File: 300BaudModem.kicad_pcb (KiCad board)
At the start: 4 copper layers, 160 x 100 mm, 27 parts, among them U1 LM7905, X2 Raw

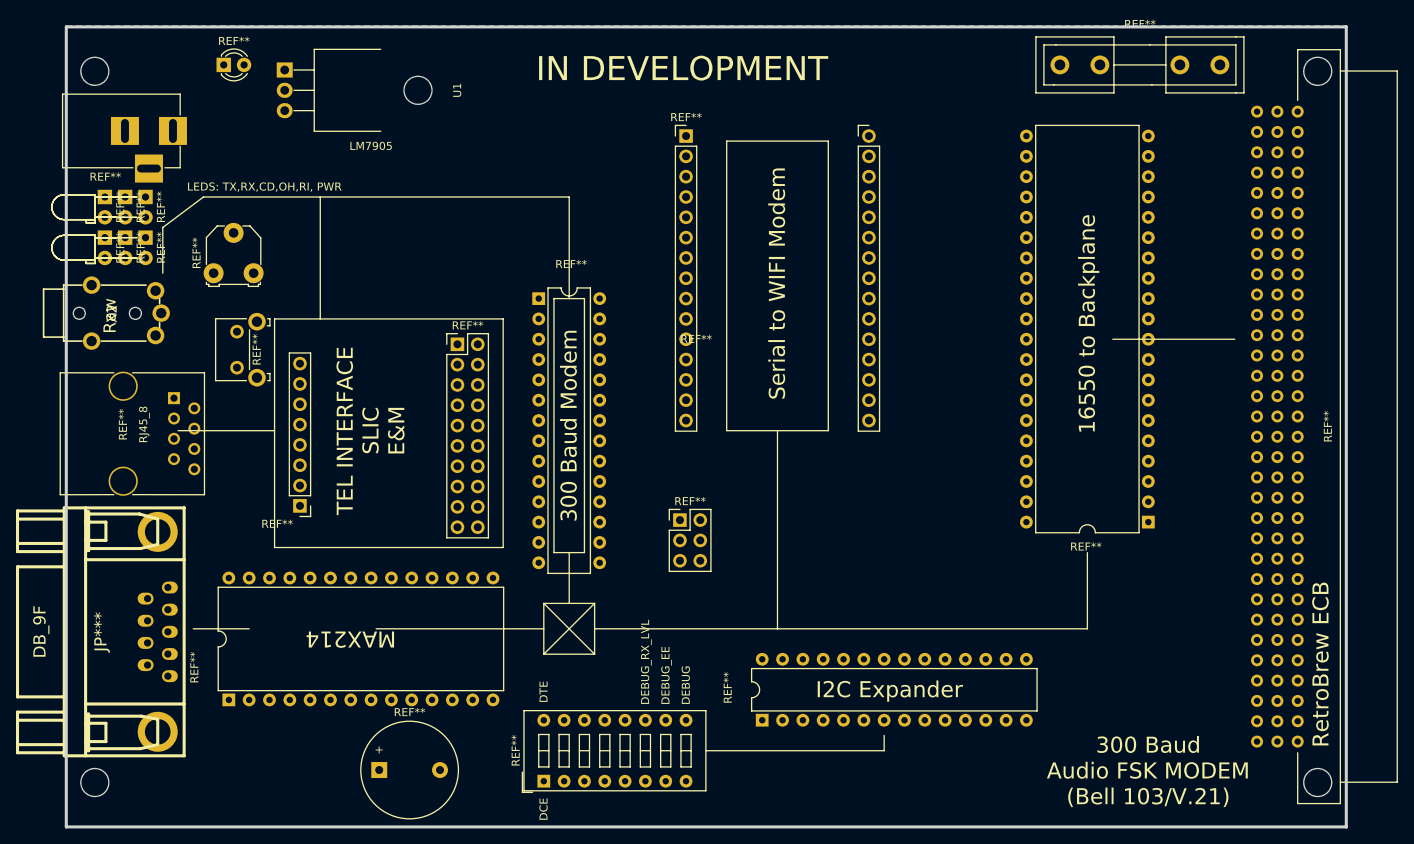
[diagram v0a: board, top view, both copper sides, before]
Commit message: updates
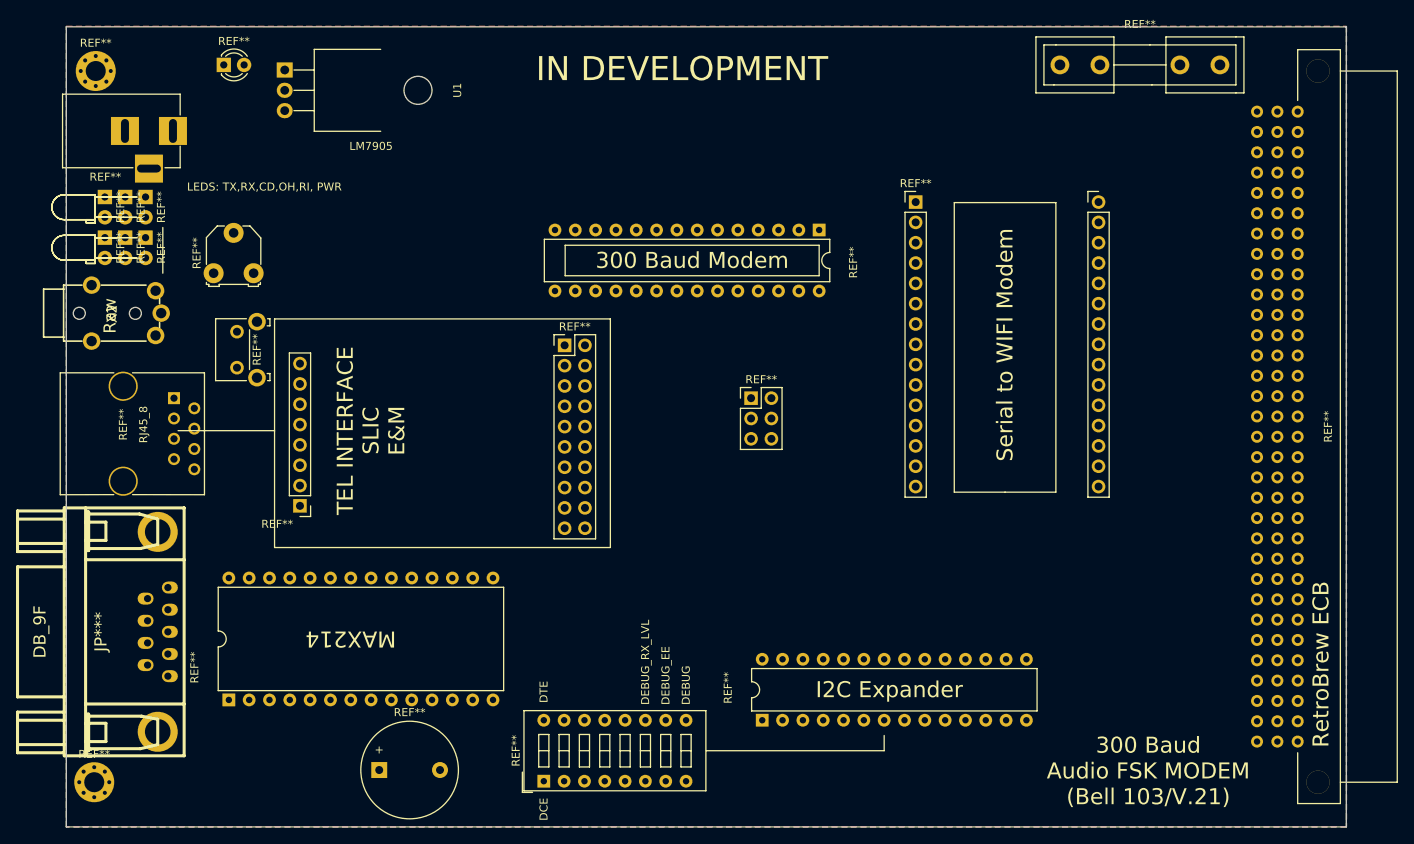
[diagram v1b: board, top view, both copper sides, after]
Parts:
- removed the REF** at (74.9, 142.2)
- removed the REF** at (210.2, 104.1)
- added REF**: MountingHole_2.5mm_Pad_Via, Mounting_Holes:MountingHole_2.5mm_Pad_Via, F.Cu at (78.6, 47.8)
- added REF**: MountingHole_2.5mm_Pad_Via, Mounting_Holes:MountingHole_2.5mm_Pad_Via, F.Cu at (78.4, 136.7)
- moved REF** 36.1 mm to (169.0, 67.6), turned to 270 degrees
- moved REF** 29.9 mm to (181.1, 64.1)
- moved REF** 17.6 mm to (160.5, 88.6)
- moved REF** 13.4 mm to (137.2, 82.0)
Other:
- board text removed: "16550 to Backplane"
